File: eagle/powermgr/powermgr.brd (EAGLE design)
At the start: 100 x 80 mm, 18 parts, among them IC1 PIC16F1455, IC2 4027D, IC3 MCP1703DB, Q1 BSS123, Q2 BSS123, X1 MINI-USB-32005-201

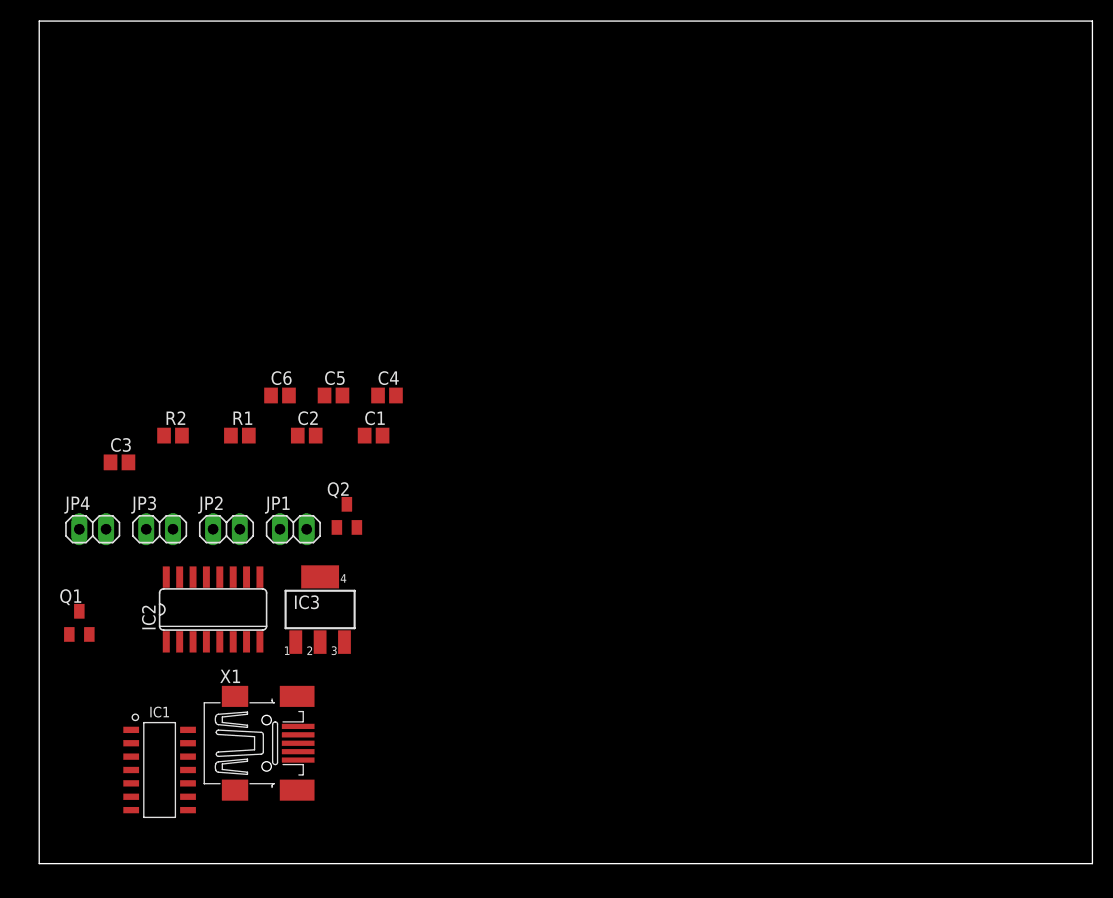
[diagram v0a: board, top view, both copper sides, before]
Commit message: First pass of power management board completed
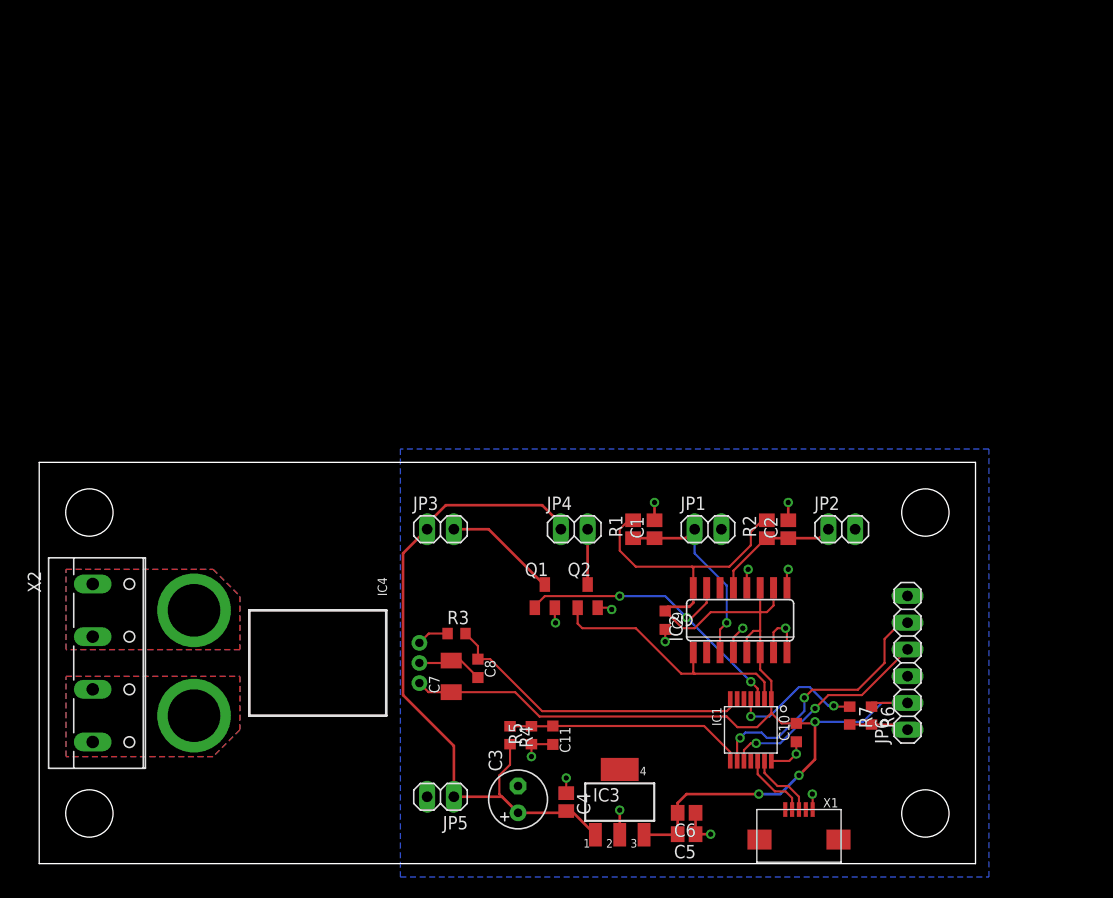
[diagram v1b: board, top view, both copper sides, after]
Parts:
- added C10, C9: .1u, resistor:C0603K
- added C11, C8: 10n, resistor:C0603K
- added C7: 0.1u, resistor:C1206K
- added IC4: ACS756, custom:5PFF
- added JP5: (no value), pinhead:1X02
- added JP6: (no value), pinhead:1X06
- added R3: 1k, resistor:R0603
- added R4: 50k, resistor:R0603
- added R5, R6: 10k, resistor:R0603
- added R7: 220, resistor:R0603
- added X2: (no value), con-wago-500:W237-4
- C3: value (none) -> 47u; device resistor:C0805 -> resistor:E2,5-6
- C4, C5: value (none) -> .1u
- C6: value (none) -> 1u
- IC1: value PIC16F1455 -> PIC16F1455TSSOP-14; device custom:SOIC-14 -> custom:TSSOP-14
- IC3: value MCP1703DB -> MCP1804
- X1: value MINI-USB-32005-201 -> 10104111-0001LF; device con-cypressindustries:32005-201 -> custom:USBAB
- moved JP2 58.4 mm to (76.2, 31.8)
- moved R2 57.1 mm to (69.1, 31.8), turned to 90 degrees
- moved IC1 56.3 mm to (67.6, 12.7), turned to 270 degrees
- moved C6 55.3 mm to (61.5, 4.83), turned to 180 degrees
- moved C5 53.5 mm to (61.5, 2.79), turned to 180 degrees
- moved X1 51.4 mm to (72.1, 2.29)
- moved IC2 50.0 mm to (66.5, 23.1)
- moved C3 49.6 mm to (45.5, 6.10), turned to 90 degrees
- moved C2 46.6 mm to (71.1, 31.8), turned to 90 degrees
- moved JP4 45.7 mm to (50.8, 31.8)
- moved Q1 44.3 mm to (48.0, 25.4)
- moved C4 42.2 mm to (50.0, 5.84), turned to 270 degrees
- moved JP1 39.4 mm to (63.5, 31.8)
- moved R1 38.4 mm to (56.4, 31.8), turned to 90 degrees
- moved IC3 33.8 mm to (55.1, 5.84)
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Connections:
- new net CURRENT: C8.1, IC1.7, R3.2
- new net N$10: C11.1, IC1.8, R4.1, R5.2
- new net N$11: JP6.1, R6.2, R7.2
- new net N$5: IC4.4, X2.1, X2.2
- new net N$6: IC4.5, X2.3, X2.4
- new net N$9: IC4.3, R3.1
- net !MCLR: now also R7.1
- net +24V: now also C3.+, JP5.1, R4.2; no longer C3.2
- net +5V: now also C10.2, C7.1, C9.1, IC4.1, JP6.2, R6.1; no longer X1.1
- net GND: now also C10.1, C11.2, C3.-, C7.2, C8.2, C9.2, IC4.2, JP5.2, JP6.3, R5.1; no longer C3.1
- net ICSPCLK: now also JP6.5
- net ICSPDAT: now also JP6.4
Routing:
- net +5V: track 0.00 -> 134.3 mm, vias 0 -> 3
- net +24V: track 0.00 -> 66.3 mm
- net GND: track 0.00 -> 41.4 mm, vias 0 -> 15
- net PWR: track 0.00 -> 30.2 mm, vias 0 -> 3
- net CURRENT: track 0.00 -> 29.9 mm
- net ICSPCLK: track 0.00 -> 25.2 mm, vias 0 -> 2
- net KILL: track 0.00 -> 25.2 mm
- net N$10: track 0.00 -> 22.8 mm
- net ICSPDAT: track 0.00 -> 20.5 mm, vias 0 -> 2
- net N$1: track 0.00 -> 19.4 mm, vias 0 -> 1
- net !MCLR: track 0.00 -> 13.0 mm, vias 0 -> 2
- net N$2: track 0.00 -> 12.3 mm
- net N$3: track 0.00 -> 10.8 mm
- net USBD-: track 0.00 -> 6.56 mm
- net USBD+: track 0.00 -> 6.56 mm
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- added copper zone on layer 16, net GND
- added copper zone on layer 1, net N$5
- added copper zone on layer 16, net N$5
- added copper zone on layer 1, net N$6
- added copper zone on layer 16, net N$6
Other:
- board size 100 x 80 mm -> 88.9 x 38.1 mm
